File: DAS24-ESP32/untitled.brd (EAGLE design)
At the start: 153 x 83 mm, 248 parts, among them IC1 MCP23017SS, IC4 MCP23017SS, J1 10118193-0001LF, K1 SRD-05VDC-SL-C, Q1 S9013, Q2 12MHz, Q3 MMBT3904, Q4 MMBT3904, Q5 S9013, Q6 S9013, U1 CH340G, U2 AMS1117, U3 ESP32-WROOM-32D, U4 PC817X2NIP0F, U49 PC817X2NIP0F, U5 PC817X2NIP0F, X1 MSTBA12, X2 MSTBA12, X5 MSTBA3, X6 MSTBA3, X7 MSTBA2, X8 MSTBA2

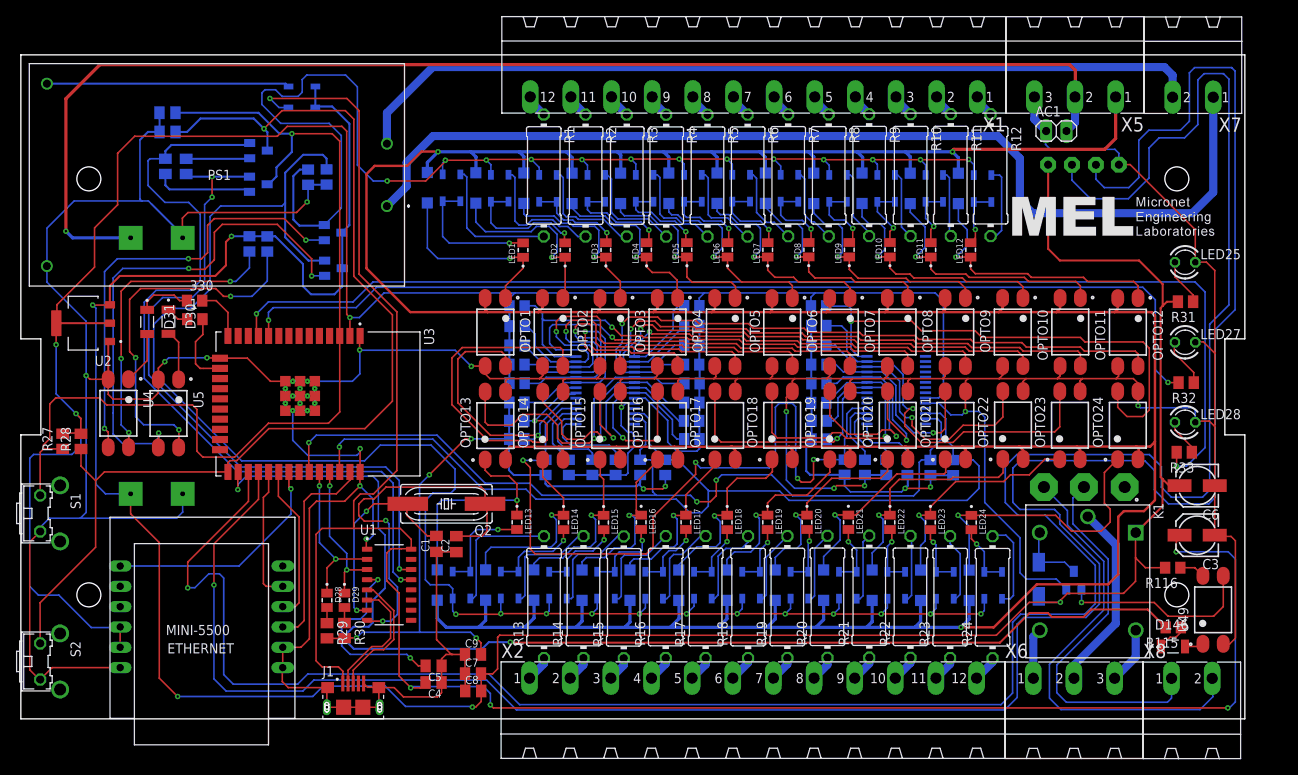
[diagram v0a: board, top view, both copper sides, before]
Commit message: pengajuan das dan revisi 21/02/2023
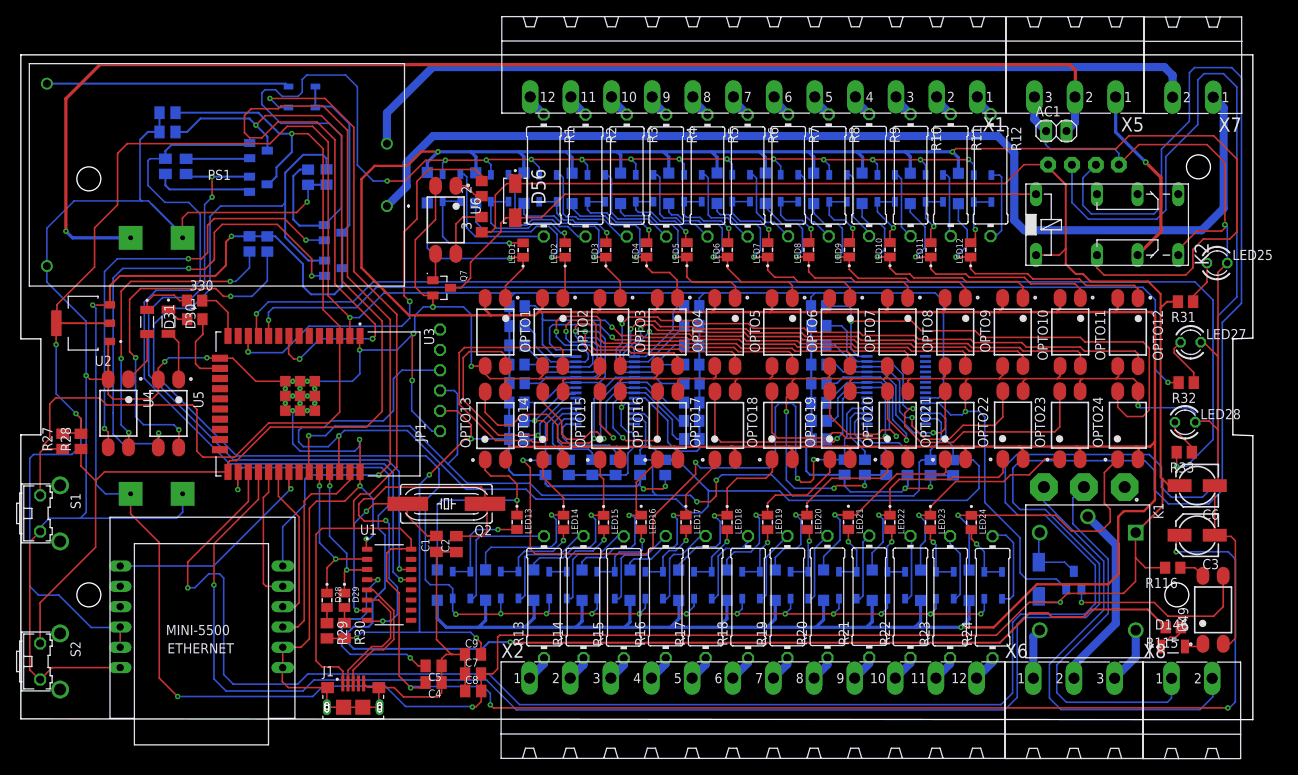
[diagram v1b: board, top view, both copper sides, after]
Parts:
- added 2: 330, rcl:R0805
- added 3: 10k, rcl:R0805
- added D56: US1M-13, US1M-13:DIOM5226X240N
- added JP1: (no value), adafruit:1X06-CLEAN
- added K2: 351, relay:351
- added Q7: S9013, S9013:SOT95P240X120-3N
- added U6: PC817X2NIP0F, PC817X2NIP0F:SOT254P975X400-4N
- 1: value (none) -> 330
- moved LED25 4.00 mm to (160.2, 65.3)
- moved LED27 0.70 mm to (156.9, 55.4)
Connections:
- new net COMM1: K2.P1, OPTO1.2, OPTO10.2, OPTO11.2, OPTO12.2, OPTO13.2, OPTO14.2, OPTO15.2, OPTO16.2, OPTO17.2, OPTO18.2, OPTO19.2, OPTO2.2, OPTO20.2, OPTO21.2, OPTO22.2, OPTO23.2, OPTO24.2, OPTO3.2, OPTO4.2, OPTO5.2, OPTO6.2, OPTO7.2, OPTO8.2, OPTO9.2, Z1.A, Z10.A, Z11.A, Z12.A, Z13.A, Z14.A, Z15.A, Z16.A, Z17.A, Z18.A, Z19.A, Z2.A, Z20.A, Z21.A, Z22.A, Z23.A, Z24.A, Z3.A, Z4.A, Z5.A, Z6.A, Z7.A, Z8.A, Z9.A
- new net GND_TEST: 2.2, U3.12
- new net INT_LAN: U$1.INT, U3.8
- new net N$14: 2.1, U6.1
- new net N$18: 3.2, U6.4
- new net N$23: D56.A, K2.16, Q7.3
- new net N$25: Q7.1, U6.3
- net COMM: now also K2.O1; no longer OPTO1.2, OPTO10.2, OPTO11.2, OPTO12.2, OPTO13.2, OPTO14.2, OPTO15.2, OPTO16.2, OPTO17.2, OPTO18.2, OPTO19.2, OPTO2.2, OPTO20.2, OPTO21.2, OPTO22.2, OPTO23.2, OPTO24.2, OPTO3.2, OPTO4.2, OPTO5.2, OPTO6.2, OPTO7.2, OPTO8.2, OPTO9.2, Z1.A, Z10.A, Z11.A, Z12.A, Z13.A, Z14.A, Z15.A, Z16.A, Z17.A, Z18.A, Z19.A, Z2.A, Z20.A, Z21.A, Z22.A, Z23.A, Z24.A, Z3.A, Z4.A, Z5.A, Z6.A, Z7.A, Z8.A, Z9.A
- net GND: now also JP1.1, K2.S1, Q7.2, U6.2
- net OUT+: now also 3.1, D56.C, K2.1
- net SCL: now also JP1.4
- net SDA: now also JP1.3
- net VCC: now also JP1.2
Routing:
- net COMM1: track 0.00 -> 587.3 mm, vias 0 -> 3
- net COMM: track 542.4 -> 23.3 mm, vias 3 -> 1
- net INT_LAN: track 0.00 -> 138.6 mm, vias 0 -> 3
- net OUT+: track 336.6 -> 416.5 mm
- net N$23: track 0.00 -> 79.9 mm
- net GND: track 661.8 -> 722.9 mm, vias 15 -> 19
- net GND_TEST: track 0.00 -> 51.8 mm, vias 0 -> 2
- net SCL: track 120.7 -> 152.7 mm
- net SDA: track 112.7 -> 125.8 mm
- net RX-RS485: track 292.8 -> 301.2 mm
- net N$18: track 0.00 -> 7.31 mm
- net L: track 128.7 -> 135.4 mm
- net TX-RS485: track 298.3 -> 304.6 mm
- net UJIDEVICE00: track 213.6 -> 207.8 mm
- net VCC: track 419.3 -> 423.6 mm
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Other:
- board size 153 x 83 mm -> 154 x 83.1 mm
